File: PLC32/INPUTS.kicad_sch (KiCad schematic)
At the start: 30 parts, among them J10 Conn_01x04, J2 Conn_01x04, J7 Conn_01x04, J8 Conn_01x04, J9 Conn_01x04, U2 PC817, U3 PC817, U4 PC817, U5 PC817, U6 PC817

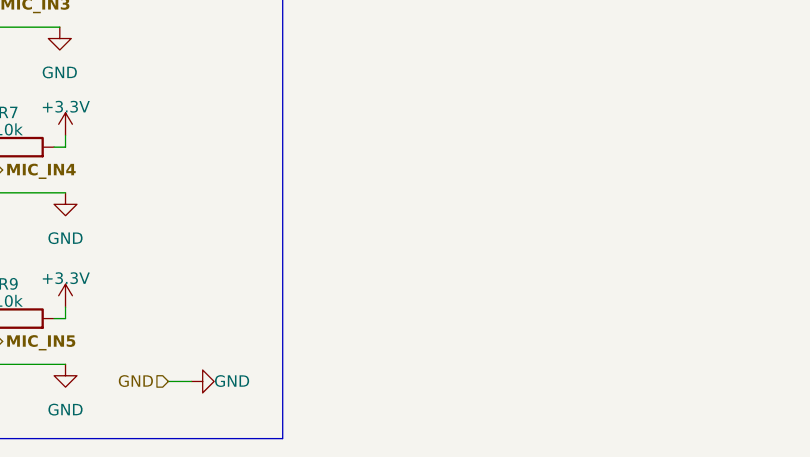
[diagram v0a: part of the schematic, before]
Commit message: adicionado diodo de alimentação das entradas digitais
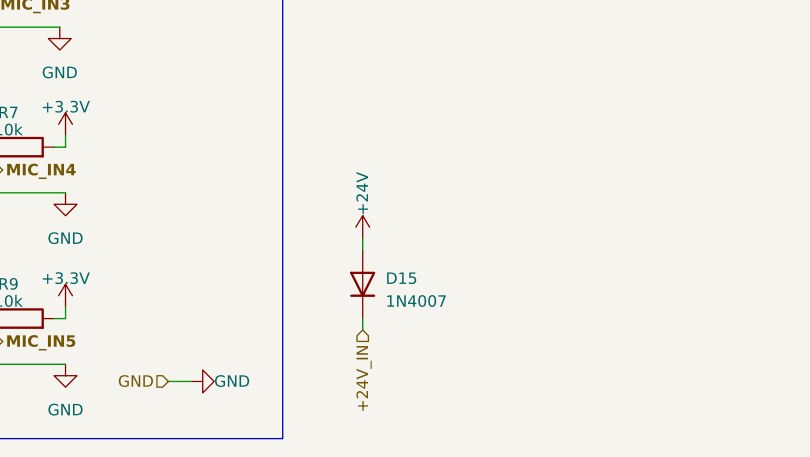
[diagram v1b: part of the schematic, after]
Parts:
- added D15: 1N4007, Diode_SMD:D_SMA, symbol Diode:1N4007
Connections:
- net +24V: now also D15.2 (A)
- new net +24V_IN: D15.1 (K)
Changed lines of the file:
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@@
     (stroke (width 0) (type default))
   )
+  (wire (pts (xy 204.47 111.76) (xy 204.47 113.03))
+    (stroke (width 0) (type default))
+  )
   (wire (pts (xy 128.27 64.77) (xy 128.905 64.77))
     (stroke (width 0) (type default))
@@
     (stroke (width 0) (type default))
   )
+  (wire (pts (xy 204.47 120.65) (xy 204.47 121.92))
+    (stroke (width 0) (type default))
+  )
   (wire (pts (xy 120.015 125.73) (xy 120.015 123.19))
     (stroke (width 0) (type default))
@@
     (effects (font (size 1.27 1.27) bold) (justify left))
   )
+  (hierarchical_label "+24V_IN" (shape input) (at 204.47 121.92 270) (fields_autoplaced)
+    (effects (font (size 1.27 1.27)) (justify right))
+  )
   (hierarchical_label "GND" (shape input) (at 182.88 127.635 180) (fields_autoplaced)
     (effects (font (size 1.27 1.27)) (justify right))
@@
     )
   )
+  (symbol (lib_id "Diode:1N4007") (at 204.47 116.84 90) (unit 1)
+    (in_bom yes) (on_board yes) (dnp no) (fields_autoplaced)
+    (property "Reference" "D15" (at 207.01 116.205 90)
+      (effects (font (size 1.27 1.27)) (justify right))
+    )
+    (property "Value" "1N4007" (at 207.01 118.745 90)
+      (effects (font (size 1.27 1.27)) (justify right))
+    )
+    (property "Footprint" "Diode_SMD:D_SMA" (at 208.915 116.84 0)
+      (effects (font (size 1.27 1.27)) hide)
+    )
+    (property "Datasheet" "http://www.vishay.com/docs/88503/1n4001.pdf" (at 204.47 116.84 0)
+      (effects (font (size 1.27 1.27)) hide)
+    )
+    (pin "1")
+    (pin "2")
+    (instances
+      (project "PLC32"
+        (path "/e63e39d7-6ac0-4ffd-8aa3-1841a4541b55/fdb977b4-5517-4144-ba6e-5f128153b962"
+          (reference "D15") (unit 1)
+        )
+      )
+    )
+  )
   (symbol (lib_id "Device:R") (at 166.37 101.6 90) (unit 1)
     (in_bom yes) (on_board yes) (dnp no)
@@
         )
       )
+    )
+  )
+  (symbol (lib_id "power:+24V") (at 204.47 111.76 0) (unit 1)
+    (in_bom yes) (on_board yes) (dnp no)
+    (property "Reference" "#PWR063" (at 204.47 115.57 0)
+      (effects (font (size 1.27 1.27)) hide)
+    )
+    (property "Value" "+24V" (at 204.47 109.22 90)
+      (effects (font (size 1.27 1.27)) (justify left))
+    )
+    (property "Footprint" "" (at 204.47 111.76 0)
+      (effects (font (size 1.27 1.27)) hide)
+    )
+    (property "Datasheet" "" (at 204.47 111.76 0)
+      (effects (font (size 1.27 1.27)) hide)
+    )
+    (pin "1")
+    (instances
+      (project "PLC32"
+        (path "/e63e39d7-6ac0-4ffd-8aa3-1841a4541b55/fdb977b4-5517-4144-ba6e-5f128153b962"
+          (reference "#PWR063") (unit 1)
+        )
+      )

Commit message: alterado diodo de alimentação das entradas digitais
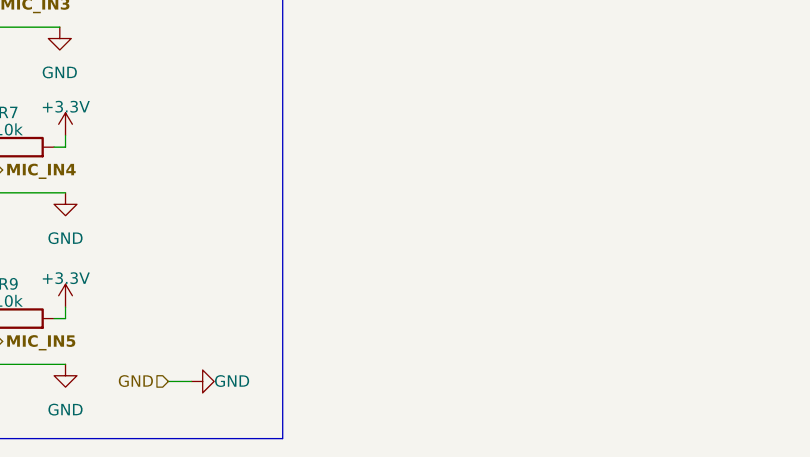
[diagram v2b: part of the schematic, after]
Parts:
- removed D15: 1N4007, Diode_SMD:D_SMA, symbol Diode:1N4007
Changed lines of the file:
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@@
     (stroke (width 0) (type default))
   )
-  (wire (pts (xy 204.47 111.76) (xy 204.47 113.03))
-    (stroke (width 0) (type default))
-  )
   (wire (pts (xy 128.27 64.77) (xy 128.905 64.77))
     (stroke (width 0) (type default))
@@
     (stroke (width 0) (type default))
   )
-  (wire (pts (xy 204.47 120.65) (xy 204.47 121.92))
-    (stroke (width 0) (type default))
-  )
   (wire (pts (xy 120.015 125.73) (xy 120.015 123.19))
     (stroke (width 0) (type default))
@@
     (effects (font (size 1.27 1.27) bold) (justify left))
   )
-  (hierarchical_label "+24V_IN" (shape input) (at 204.47 121.92 270) (fields_autoplaced)
-    (effects (font (size 1.27 1.27)) (justify right))
-  )
   (hierarchical_label "GND" (shape input) (at 182.88 127.635 180) (fields_autoplaced)
     (effects (font (size 1.27 1.27)) (justify right))
@@
     )
   )
-  (symbol (lib_id "Diode:1N4007") (at 204.47 116.84 90) (unit 1)
-    (in_bom yes) (on_board yes) (dnp no) (fields_autoplaced)
-    (property "Reference" "D15" (at 207.01 116.205 90)
-      (effects (font (size 1.27 1.27)) (justify right))
-    )
-    (property "Value" "1N4007" (at 207.01 118.745 90)
-      (effects (font (size 1.27 1.27)) (justify right))
-    )
-    (property "Footprint" "Diode_SMD:D_SMA" (at 208.915 116.84 0)
-      (effects (font (size 1.27 1.27)) hide)
-    )
-    (property "Datasheet" "http://www.vishay.com/docs/88503/1n4001.pdf" (at 204.47 116.84 0)
-      (effects (font (size 1.27 1.27)) hide)
-    )
-    (pin "1")
-    (pin "2")
-    (instances
-      (project "PLC32"
-        (path "/e63e39d7-6ac0-4ffd-8aa3-1841a4541b55/fdb977b4-5517-4144-ba6e-5f128153b962"
-          (reference "D15") (unit 1)
-        )
-      )
-    )
-  )
   (symbol (lib_id "Device:R") (at 166.37 101.6 90) (unit 1)
     (in_bom yes) (on_board yes) (dnp no)
@@
         )
       )
-    )
-  )
-  (symbol (lib_id "power:+24V") (at 204.47 111.76 0) (unit 1)
-    (in_bom yes) (on_board yes) (dnp no)
-    (property "Reference" "#PWR063" (at 204.47 115.57 0)
-      (effects (font (size 1.27 1.27)) hide)
-    )
-    (property "Value" "+24V" (at 204.47 109.22 90)
-      (effects (font (size 1.27 1.27)) (justify left))
-    )
-    (property "Footprint" "" (at 204.47 111.76 0)
-      (effects (font (size 1.27 1.27)) hide)
-    )
-    (property "Datasheet" "" (at 204.47 111.76 0)
-      (effects (font (size 1.27 1.27)) hide)
-    )
-    (pin "1")
-    (instances
-      (project "PLC32"
-        (path "/e63e39d7-6ac0-4ffd-8aa3-1841a4541b55/fdb977b4-5517-4144-ba6e-5f128153b962"
-          (reference "#PWR063") (unit 1)
-        )
-      )
